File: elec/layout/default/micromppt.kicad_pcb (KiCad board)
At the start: 2 copper layers, 25.9 x 15.3 mm, 18 parts, among them U6 10kΩ ±1% 62.5mW

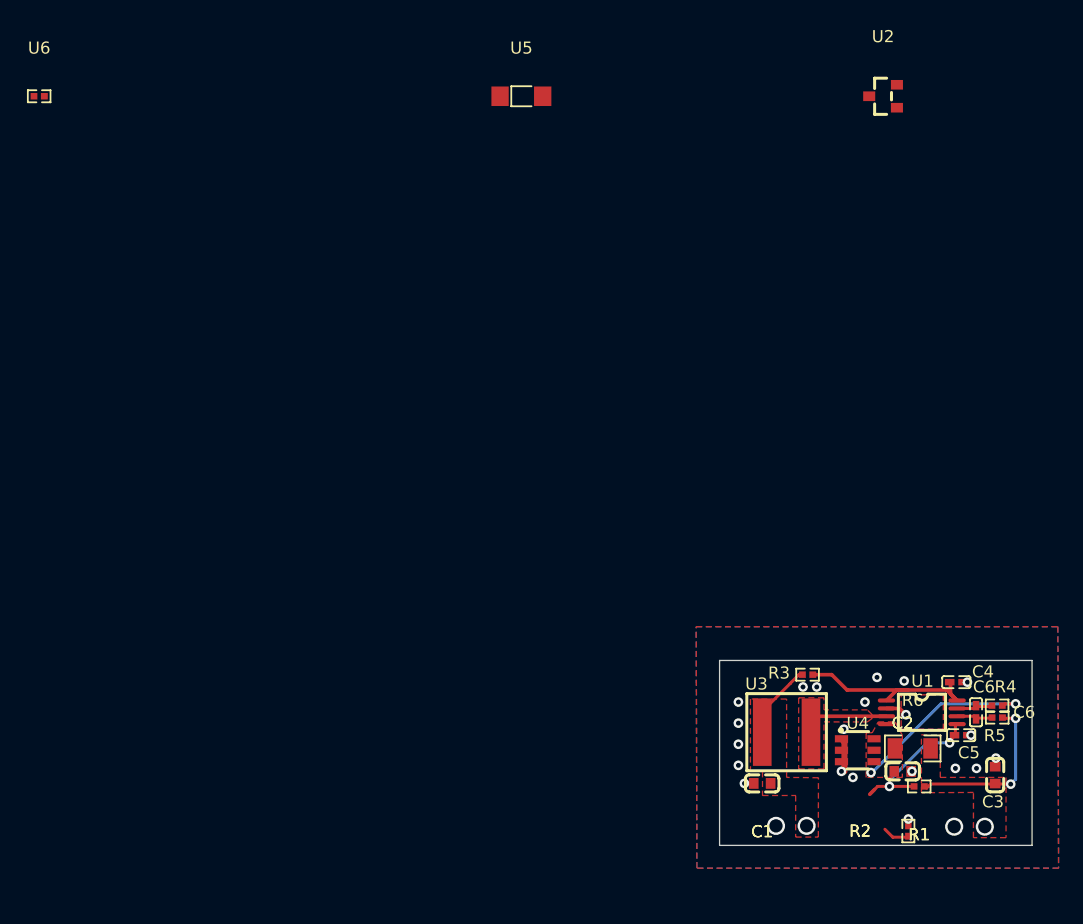
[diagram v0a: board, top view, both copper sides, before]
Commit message: Micromppt V3 (fr this time)
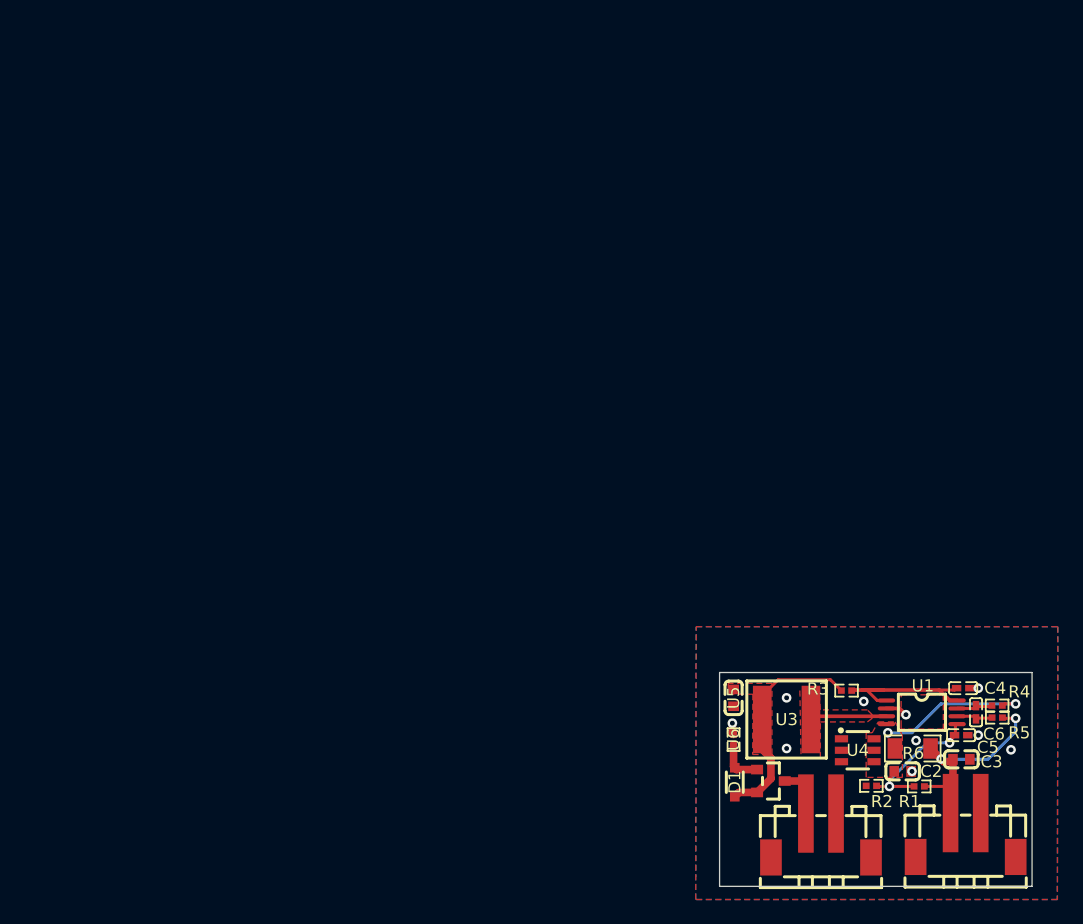
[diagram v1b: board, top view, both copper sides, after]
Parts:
- removed C1: 10µF ±10% 10V X5R, atopile:C0603-bd72f6
- added D1: , lib:SOD-323F_L1.7-W1.3-LS2.5-R-RD, F.Cu at (67.7, 51.9)
- added U7: , lib:CONN-SMD_2P-P2.50_DEALON_XH-2PS, F.Cu at (86.8, 56.3)
- added U8: , lib:CONN-SMD_2P-P2.50_DEALON_XH-2PS, F.Cu at (74.8, 56.3)
- U5: value (none) -> 10µF ±10% 10V X5R; footprint lib:SOD-80_L3.5-W1.5-RD -> atopile:C0603-bd72f6
- moved U6 78.5 mm to (67.6, 48.4), turned to 90 degrees
- moved U2 57.6 mm to (70.7, 51.8), turned to 180 degrees
- moved U5 52.9 mm to (67.6, 44.9), turned to -90 degrees
- moved R2 4.85 mm to (79.0, 52.2), turned to 180 degrees
- moved R3 3.49 mm to (77.0, 44.3)
- moved C3 3.09 mm to (86.5, 50.0), turned to 0 degrees
- moved U3 1.05 mm to (72.0, 46.7)
- moved C4 0.76 mm to (86.7, 44.1)
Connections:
- net S renamed C
- U2 pad 1: G -> A
- U4 pad 1: gnd -> (no net)
- U4 pad 2: gnd -> (no net)
- U4 pad 3: gnd -> (no net)
- U5 pad 2: G -> gnd
- U6 pad 1: G -> A
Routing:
- net C: track 0.00 -> 21.8 mm
- net (no net): track 21.7 -> 0.00 mm, vias 3 -> 0
- net VCTRL: track 0.00 -> 11.5 mm, vias 0 -> 2
- net hv: track 13.9 -> 20.4 mm, vias 3 -> 2
- net D: track 0.00 -> 4.27 mm
- net A: track 0.00 -> 3.85 mm
- net VOUT: track 15.4 -> 12.7 mm
- net net: track 2.22 -> 0.00 mm
- net gnd: track 4.64 -> 2.81 mm, vias 23 -> 10
- net XSHUT: track 16.7 -> 15.5 mm
- added copper zone on F.Cu, net C
- removed copper zone on F.Cu, net hv
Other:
- board size 25.9 x 15.3 mm -> 25.9 x 17.7 mm

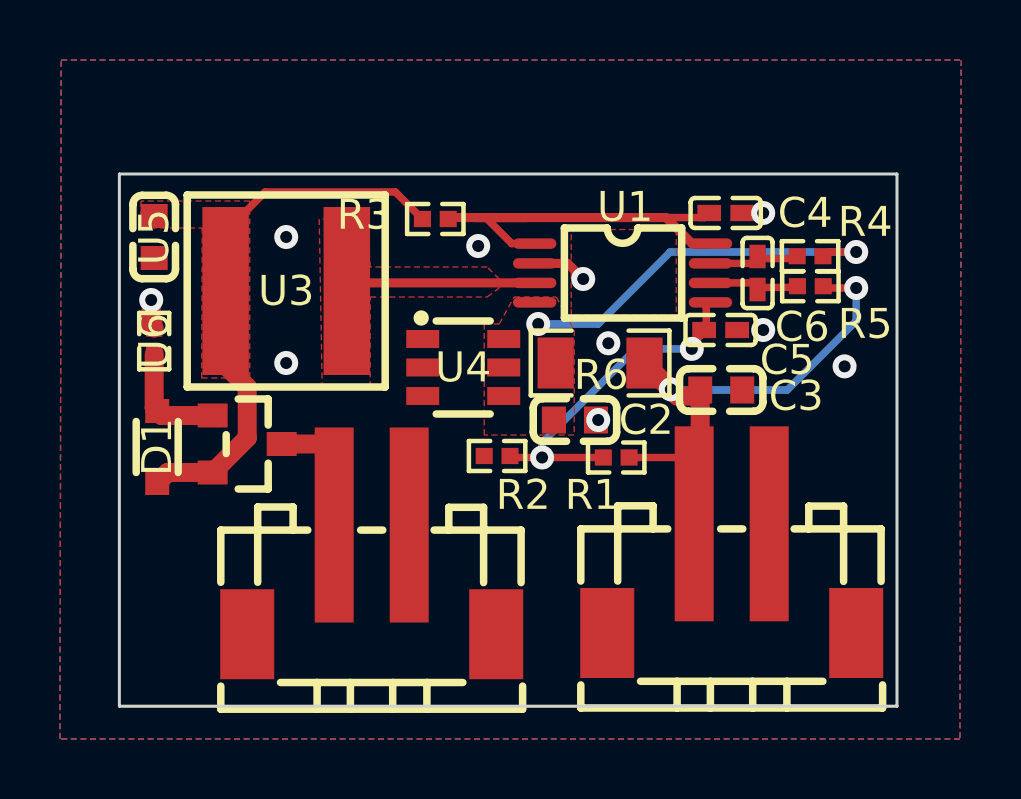
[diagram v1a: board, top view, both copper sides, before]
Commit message: Micromppt V3 (fr this time) x2
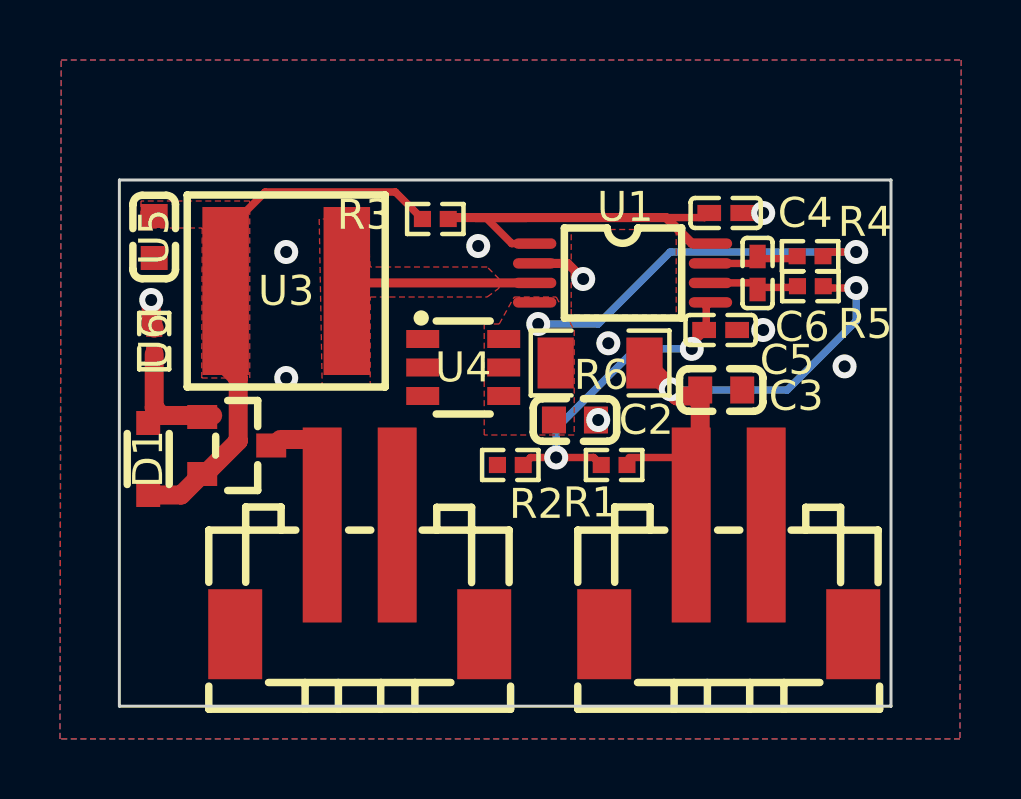
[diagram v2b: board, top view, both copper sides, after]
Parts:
- moved R2 0.53 mm to (79.5, 52.5)
- moved D1 0.50 mm to (67.4, 52.3)
- moved U8 0.40 mm to (74.5, 56.3)
- moved U2 0.35 mm to (70.3, 51.9)
- moved R1 0.26 mm to (82.9, 52.5)
- moved U7 0.11 mm to (86.8, 56.3)
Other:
- board size 25.9 x 17.7 mm -> 25.7 x 17.5 mm
